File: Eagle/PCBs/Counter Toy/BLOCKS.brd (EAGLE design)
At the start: 6 parts, among them U1 MC74HC1G14DTT1G

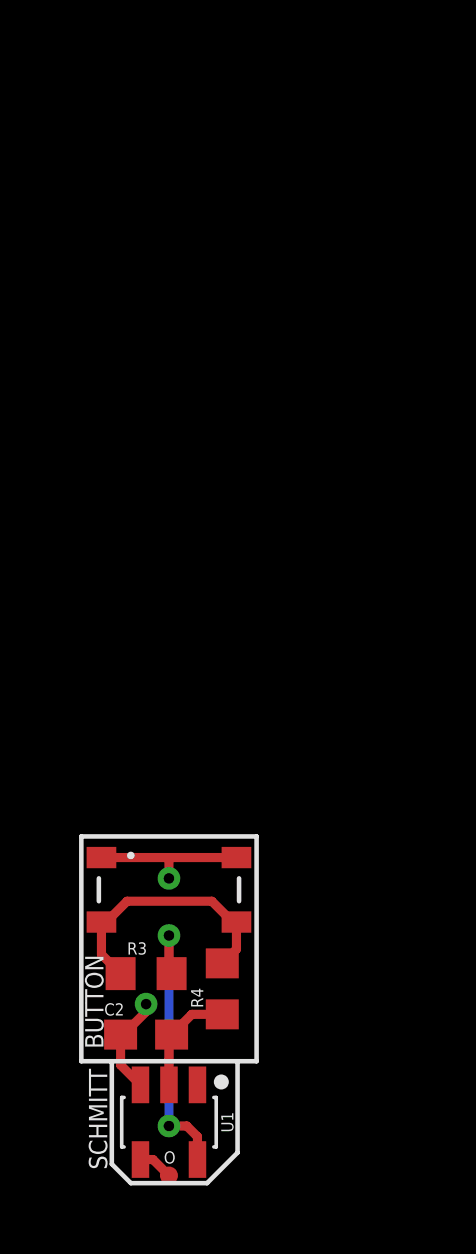
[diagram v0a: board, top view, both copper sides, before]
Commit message: Better DFF
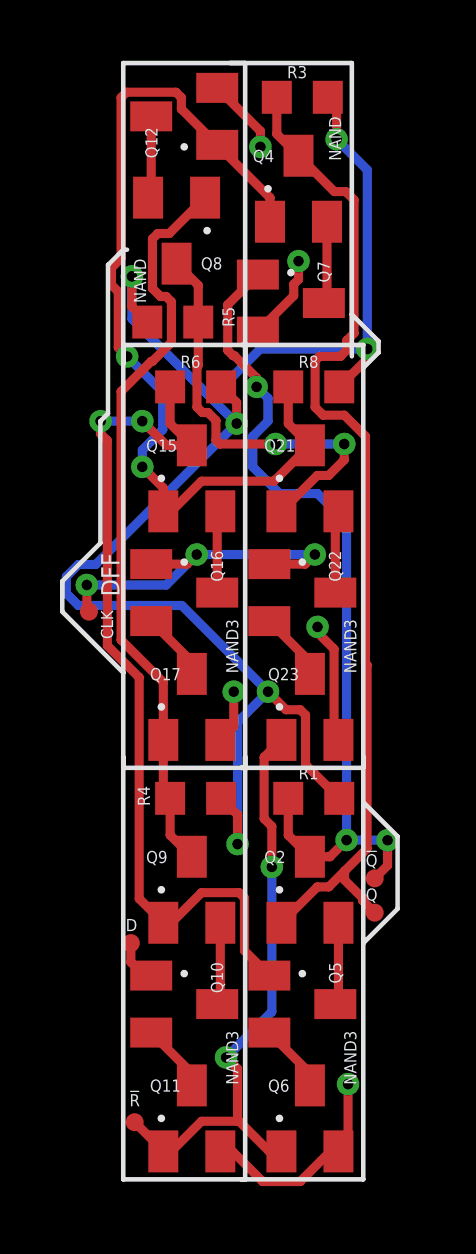
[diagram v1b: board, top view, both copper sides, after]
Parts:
- removed C2: 0.1u, ellajameson-core:C0603
- removed O: TPPAD6, ellajameson-core:TP06R
- removed S2: (no value), ellajameson-core:SW4_PTS815_SJM_250_SMTR_LFS_CN
- removed U1: MC74HC1G14DTT1G, ellajameson-core:SOT95P275X110-5N
- added !Q, !R, CLK, D, Q: TPPAD6, ellajameson-core:TP06R
- added Q10, Q11, Q12, Q15, Q16, Q17, Q2, Q21, Q22, Q23, Q4, Q5, Q6, Q7, Q8, Q9: 2N7002, ellajameson-core:SOT23
- added R1, R5, R6, R8: (no value), ellajameson-core:R0603
- R3, R4: value 10k -> (none)
- moved R3 29.7 mm to (7.24, 36.2)
- moved R4 6.41 mm to (3.68, 12.8), turned to 0 degrees
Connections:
- removed net N$1: O.TP, U1.4
- removed net N$3: R3.1, R4.2, S2.3, S2.4
- new net N$10: Q2.2, Q5.3
- new net N$12: Q5.2, Q6.3
- new net N$14: Q4.2, Q7.3
- new net N$16: Q21.1, Q8.3, R5.1
- new net N$18: Q17.1, Q8.1, Q9.3, R4.1
- new net N$19: D.TP, Q10.1
- new net N$20: Q10.3, Q9.2
- new net N$22: Q10.2, Q11.3
- new net N$24: Q12.3, Q8.2
- new net N$31: CLK.TP, Q16.1, Q22.1
- new net N$32: Q15.2, Q16.3
- new net N$34: Q16.2, Q17.3
- new net N$44: Q21.2, Q22.3
- new net N$45: !R.TP, Q11.1, Q23.1, Q6.1
- new net N$46: Q22.2, Q23.3
- new net N$7: Q12.1, Q15.1, Q21.3, Q4.1, R8.1
- new net N$8: Q.TP, Q2.1, Q4.3, R3.1
- new net N$9: Q15.3, Q5.1, Q9.1, R6.1
- net GND: now also Q11.2, Q12.2, Q17.2, Q23.2, Q6.2, Q7.2; no longer C2.2, S2.1, S2.2, U1.3
- net N$4: now also !Q.TP, Q2.3, Q7.1, R1.1; no longer C2.1, R4.1, U1.2
- net VCC: now also R1.2, R4.2, R5.2, R6.2, R8.2; no longer U1.5
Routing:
- net VCC: track 9.52 -> 54.5 mm, vias 2 -> 6
- net N$8: track 0.00 -> 34.1 mm
- net N$7: track 0.00 -> 30.8 mm, vias 0 -> 2
- net N$9: track 0.00 -> 29.3 mm, vias 0 -> 2
- net N$18: track 0.00 -> 25.0 mm
- net N$4: track 3.68 -> 28.6 mm, vias 0 -> 3
- net N$45: track 0.00 -> 20.0 mm, vias 0 -> 2
- net N$16: track 0.00 -> 14.2 mm, vias 0 -> 2
- net N$31: track 0.00 -> 12.2 mm, vias 0 -> 3
- net GND: track 8.56 -> 18.5 mm, vias 2 -> 5
- net N$3: track 8.63 -> 0.00 mm
- net N$32: track 0.00 -> 2.75 mm
- net N$24: track 0.00 -> 2.75 mm
- net N$44: track 0.00 -> 2.75 mm
- net N$20: track 0.00 -> 2.75 mm
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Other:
- board text added: "DFF"
- board text added: "NAND"
- board text added: "NAND3"
- board text removed: "BUTTON"
- board text removed: "SCHMITT"
